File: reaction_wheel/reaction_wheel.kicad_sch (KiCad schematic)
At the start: 20 parts, among them U1 MCF8315C1VQRGFRQ1

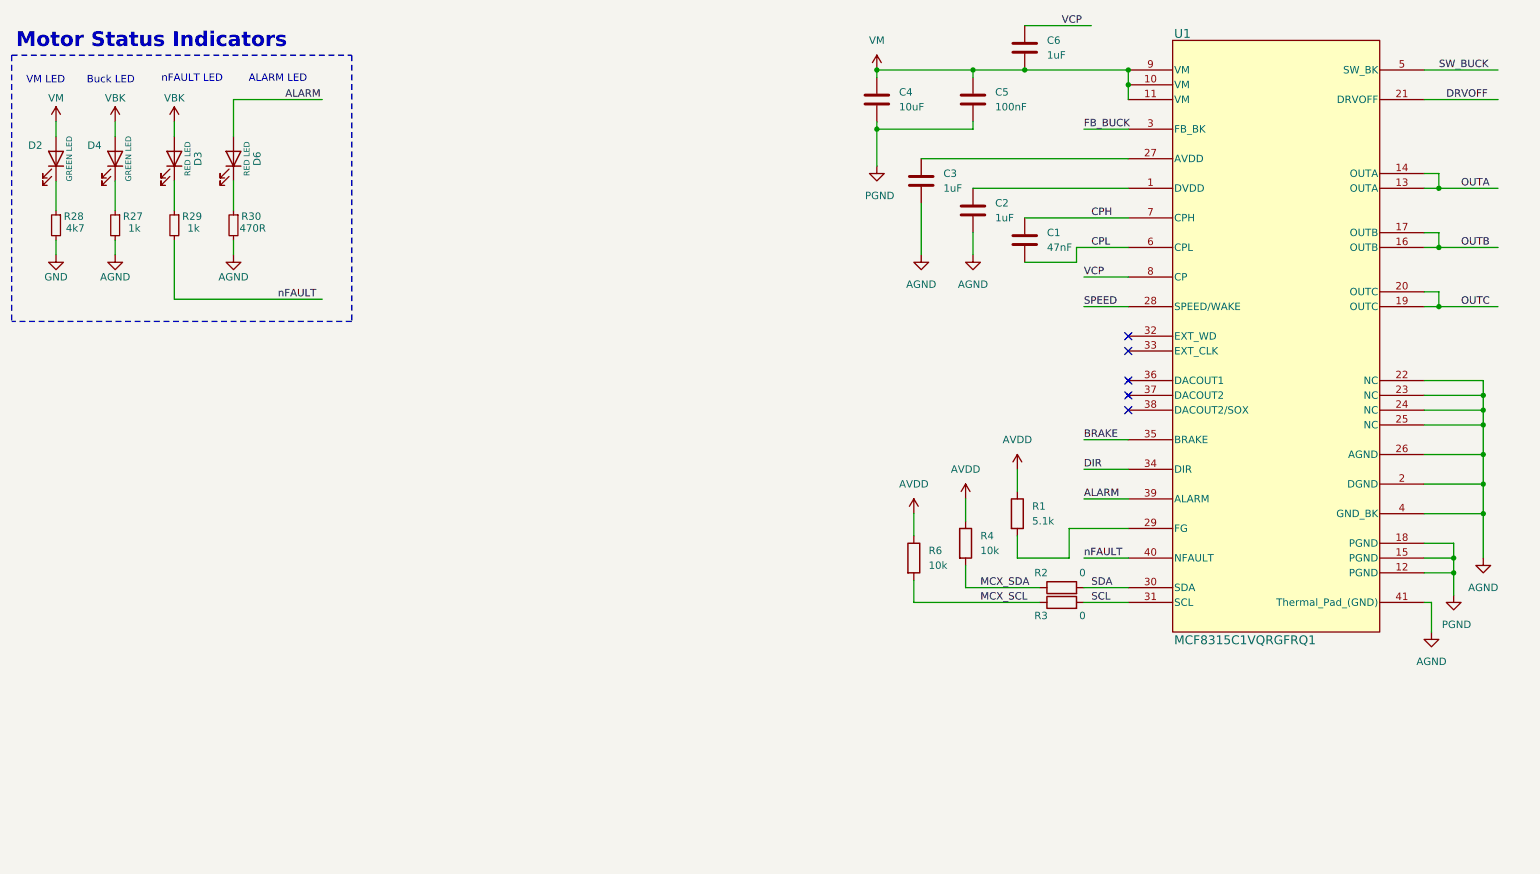
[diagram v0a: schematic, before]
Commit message: started rw baseboard
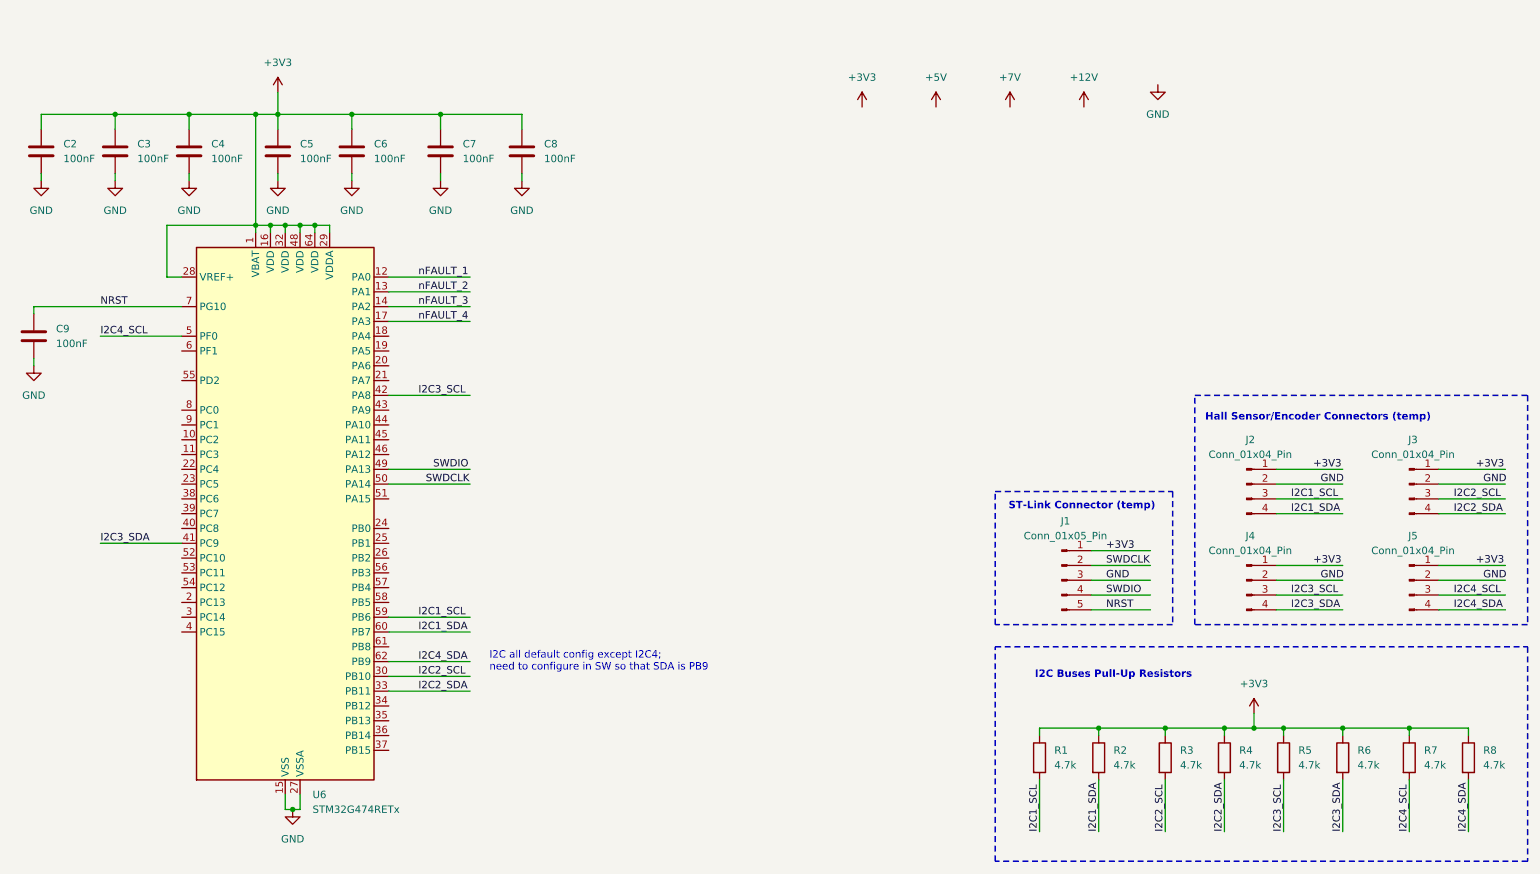
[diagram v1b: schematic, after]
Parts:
- removed C1: 47nF, symbol Device:C
- removed D2, D4: GREEN LED, LED_SMD:LED_0603_1608Metric, symbol Device:LED
- removed D3, D6: RED LED, LED_SMD:LED_0603_1608Metric, symbol Device:LED
- removed R27, R29: 1k, Resistor_SMD:R_0603_1608Metric, symbol Device:R_Small
- removed R28: 4k7, Resistor_SMD:R_0603_1608Metric, symbol Device:R_Small
- removed R30: 470R, Resistor_SMD:R_0603_1608Metric, symbol Device:R_Small
- removed U1: MCF8315C1VQRGFRQ1, Argus_RW_Library:VQFN40_RGF_TEX, symbol Argus_RW_Library:MCF8315C1VQRGFRQ1
- added C7, C8, C9: 100nF, symbol Device:C
- added J1: Conn_01x05_Pin, symbol Connector:Conn_01x05_Pin
- added J2, J3, J4, J5: Conn_01x04_Pin, symbol Connector:Conn_01x04_Pin
- added R5, R7, R8: 4.7k, symbol Device:R
- added U6: STM32G474RETx, Package_QFP:LQFP-64_10x10mm_P0.5mm, symbol MCU_ST_STM32G4:STM32G474RETx
- C2, C3, C6: value 1uF -> 100nF
- C4: value 10uF -> 100nF
- R1: value 5.1k -> 4.7k
- R2, R3: value 0 -> 4.7k
- R4, R6: value 10k -> 4.7k
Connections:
- net AGND is gone; now on net GND: C2.2, C3.2
- net AVDD is gone; now on net +3V3: R1.1, R4.1, R6.1
- net PGND is gone; now on net GND: C4.2, C5.2
- net VCP is gone; now on net +3V3: C6.1
- net GND: now also C6.2, C7.2, C8.2, C9.2, J1.3 (Pin_3), J2.2 (Pin_2), J3.2 (Pin_2), J4.2 (Pin_2), J5.2 (Pin_2), U6.15 (VSS), U6.27 (VSSA), U6.31 (VSS), U6.47 (VSS), U6.63 (VSS)
- net +3V3: now reaches C2.1
- net +3V3: now also C3.1, C4.1, C5.1, R2.1, R3.1, C7.1, C8.1, J1.1 (Pin_1), J2.1 (Pin_1), J3.1 (Pin_1), J4.1 (Pin_1), J5.1 (Pin_1), R5.1, R7.1, R8.1, U6.1 (VBAT), U6.16 (VDD), U6.28 (VREF+), U6.29 (VDDA), U6.32 (VDD), U6.48 (VDD), U6.64 (VDD)
- net I2C1_SCL: now reaches R1.2
- net I2C1_SCL: now also J2.3 (Pin_3), U6.59 (PB6)
- net MCX_SCL renamed I2C3_SDA
- net I2C3_SDA: now also J4.4 (Pin_4), U6.41 (PC9); no longer R3.1
- net MCX_SDA renamed I2C2_SDA
- net I2C2_SDA: now also J3.4 (Pin_4), U6.33 (PB11); no longer R2.1
- net SCL renamed I2C2_SCL
- net I2C2_SCL: now also J3.3 (Pin_3), U6.30 (PB10)
- net SDA renamed I2C1_SDA
- net I2C1_SDA: now also J2.4 (Pin_4), U6.60 (PB7)
- removed net VM: C4.1, C5.1, C6.2
- new net I2C3_SCL: J4.3 (Pin_3), R5.2, U6.42 (PA8)
- new net I2C4_SCL: J5.3 (Pin_3), R7.2, U6.5 (PF0)
- new net I2C4_SDA: J5.4 (Pin_4), R8.2, U6.62 (PB9)
- new net NRST: C9.1, J1.5 (Pin_5), U6.7 (PG10)
- new net SWDCLK: J1.2 (Pin_2), U6.50 (PA14)
- new net SWDIO: J1.4 (Pin_4), U6.49 (PA13)
- new net nFAULT_1: U6.12 (PA0)
- new net nFAULT_2: U6.13 (PA1)
- new net nFAULT_3: U6.14 (PA2)
- new net nFAULT_4: U6.17 (PA3)
- no-connect marks 5 -> 0
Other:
- note added: "Hall Sensor/Encoder Connectors (temp)"
- note added: "I2C Buses Pull-Up Resistors"
- note added: "I2C all default config except I2C4; need to configure in SW so that SDA is PB9"
- note added: "ST-Link Connector (temp)"
- note removed: "ALARM LED"
- note removed: "Buck LED"
- note removed: "Motor Status Indicators"
- note removed: "VM LED"
- note removed: "nFAULT LED"
